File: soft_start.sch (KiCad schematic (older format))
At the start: 21 parts, among them J10 PWR, J8 MG950-9.5, J9 MG950-9.5, K5 Fujitsu_FTR-F1C, K6 Fujitsu_FTR-F1C, Q5 BC546, Q6 BC546, U5 NE555, U6 NE555

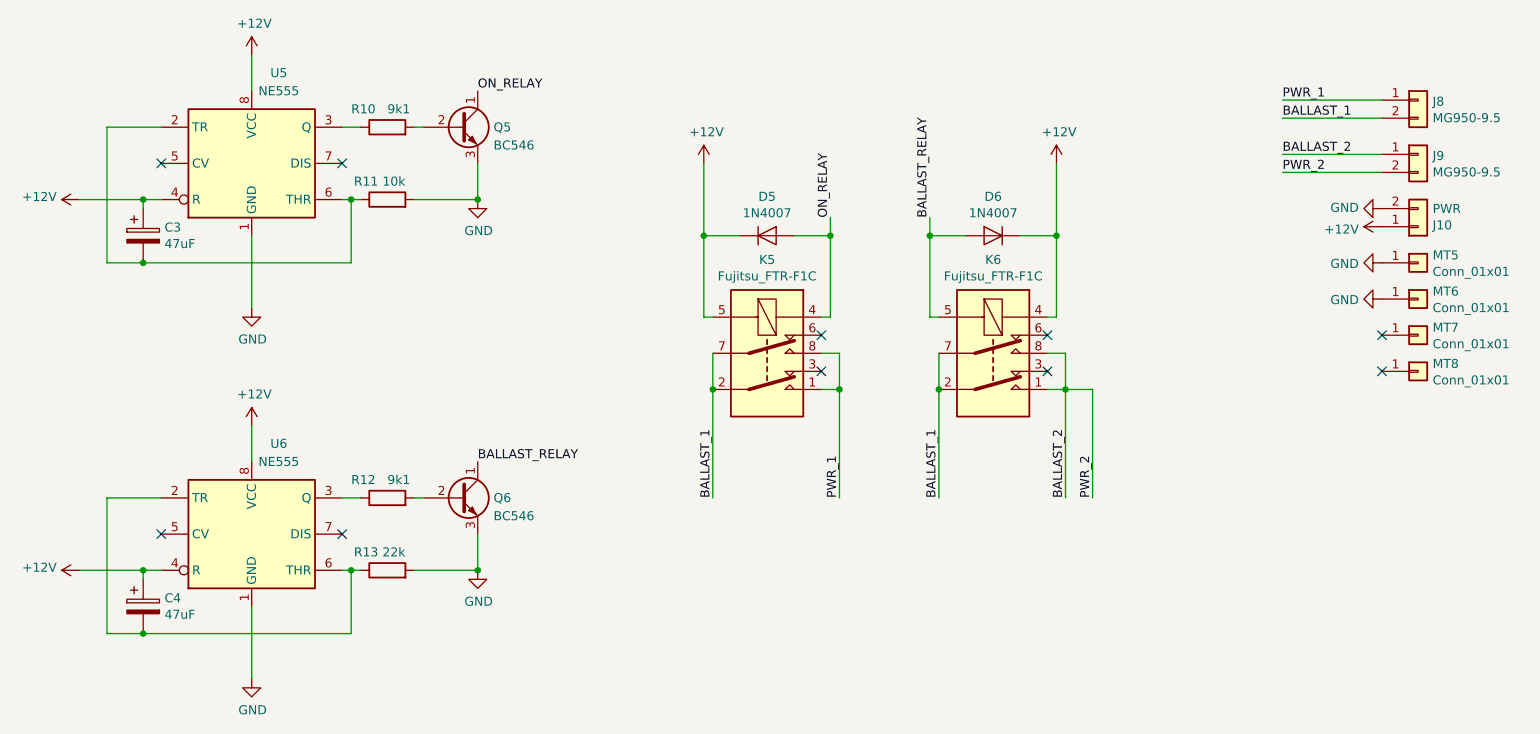
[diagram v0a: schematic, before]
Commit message: Final schematic version
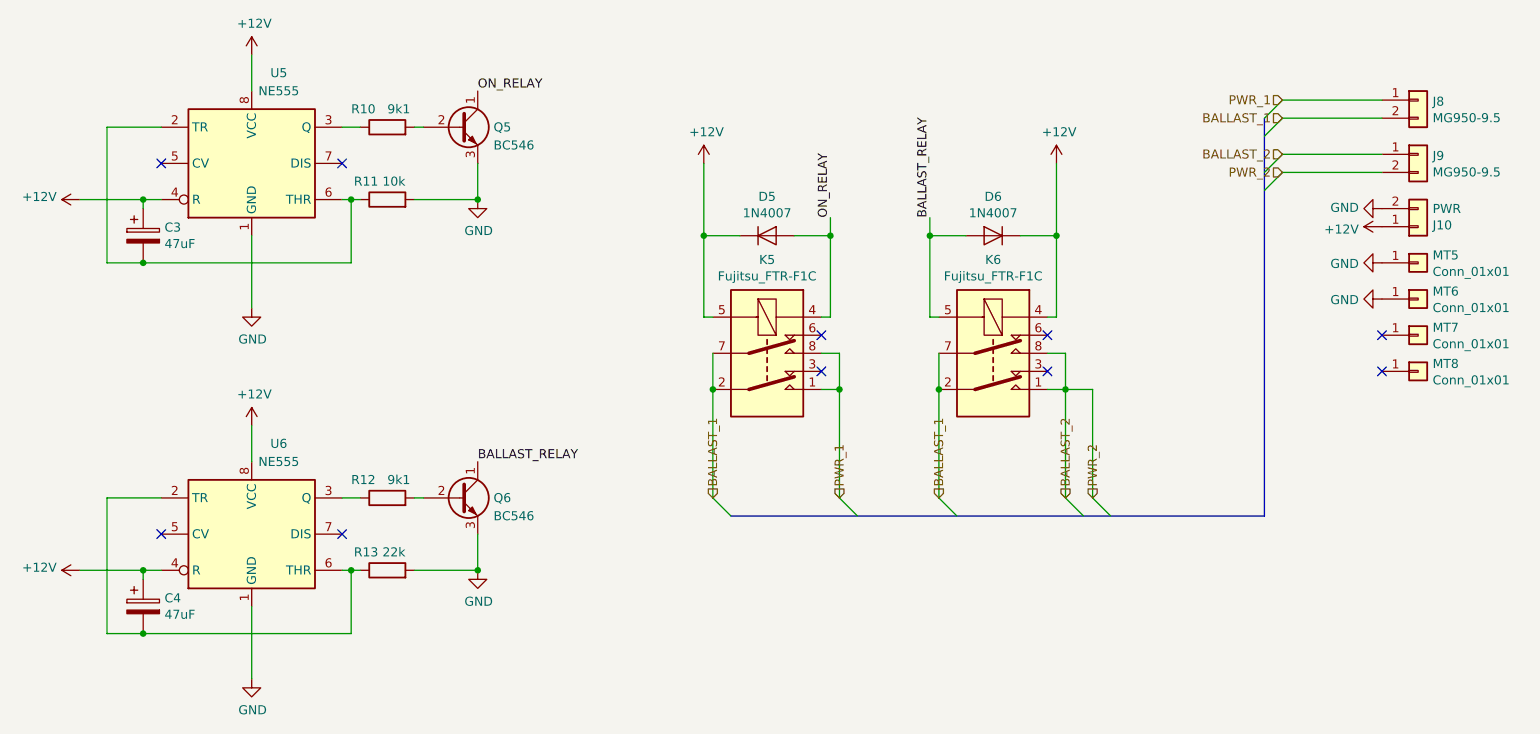
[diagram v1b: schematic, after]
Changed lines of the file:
@@
 EESchema Schematic File Version 4
 LIBS:isolation-transformer-cache
-EELAYER 26 0
+EELAYER 30 0
 EELAYER END
 $Descr A4 11693 8268
 encoding utf-8
-Sheet 3 3
+Sheet 2 3
 Title ""
 Date ""
@@
 	1    0    0    -1
 $EndComp
-Text Label 5550 3400 1    50   ~ 0
-PWR_1
-Text Label 6950 3400 1    50   ~ 0
-PWR_2
 Wire Wire Line
 	8550 1600 8000 1600
@@
 	1    0    0    -1
 $EndComp
-Text Label 8000 1500 0    50   ~ 0
-BALLAST_2
-Text Label 8000 1600 0    50   ~ 0
-PWR_2
 Wire Wire Line
 	8550 1300 8000 1300
@@
 	1    0    0    -1
 $EndComp
-Text Label 8000 1200 0    50   ~ 0
-PWR_1
-Text Label 8000 1300 0    50   ~ 0
-BALLAST_1
 Connection ~ 3550 1750
 $Comp
@@
 	1    0    0    -1
 $EndComp
-Text Label 6100 3400 1    50   ~ 0
-BALLAST_1
-Text Label 6800 3400 1    50   ~ 0
-BALLAST_2
 Text Label 6050 1850 1    50   ~ 0
 BALLAST_RELAY
@@
 Wire Wire Line
 	4850 2600 4850 2800
-Text Label 4850 3400 1    50   ~ 0
+Connection ~ 4850 2800
+Wire Wire Line
+	4850 2800 4850 3400
+Entry Wire Line
+	4850 3400 4950 3500
+Entry Wire Line
+	5550 3400 5650 3500
+Entry Wire Line
+	6100 3400 6200 3500
+Entry Wire Line
+	6800 3400 6900 3500
+Entry Wire Line
+	6950 3400 7050 3500
+Entry Wire Line
+	7900 1300 8000 1200
+Entry Wire Line
+	7900 1400 8000 1300
+Entry Wire Line
+	7900 1600 8000 1500
+Entry Wire Line
+	7900 1700 8000 1600
+Text HLabel 8000 1200 0    50   Input ~ 0
+PWR_1
+Text HLabel 8000 1300 0    50   Input ~ 0
 BALLAST_1
-Connection ~ 4850 2800
-Wire Wire Line
-	4850 2800 4850 3400
+Text HLabel 8000 1500 0    50   Input ~ 0
+BALLAST_2
+Text HLabel 8000 1600 0    50   Input ~ 0
+PWR_2
+Text HLabel 5550 3400 1    50   Input ~ 0
+PWR_1
+Text HLabel 6100 3400 1    50   Input ~ 0
+BALLAST_1
+Text HLabel 6800 3400 1    50   Input ~ 0
+BALLAST_2
+Text HLabel 6950 3400 1    50   Input ~ 0
+PWR_2
+Text HLabel 4850 3400 1    50   Input ~ 0
+BALLAST_1
+Wire Bus Line
+	4950 3500 7900 3500
+Wire Bus Line
+	7900 1300 7900 3500
 $EndSCHEMATC
